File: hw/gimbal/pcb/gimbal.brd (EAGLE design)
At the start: 60 x 40 mm, 43 parts

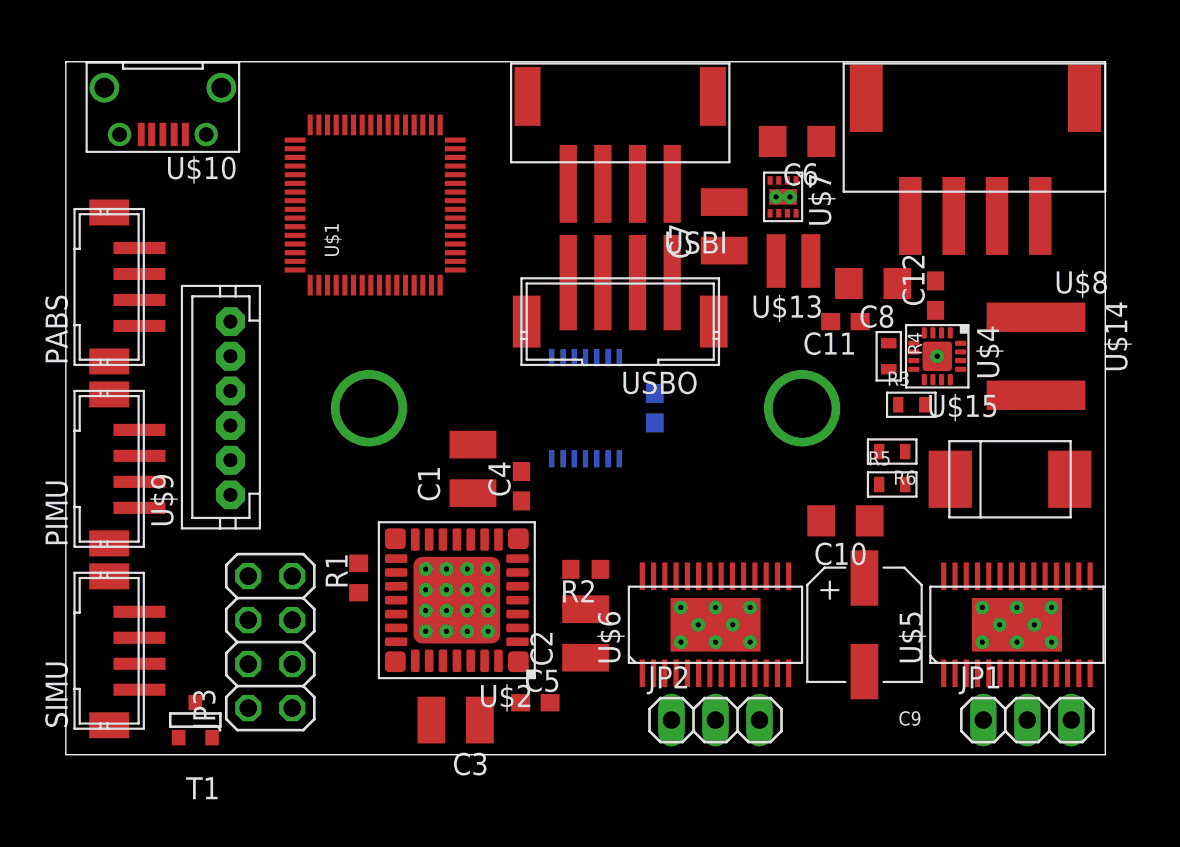
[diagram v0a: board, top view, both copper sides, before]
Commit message: Progress on gimbal board.
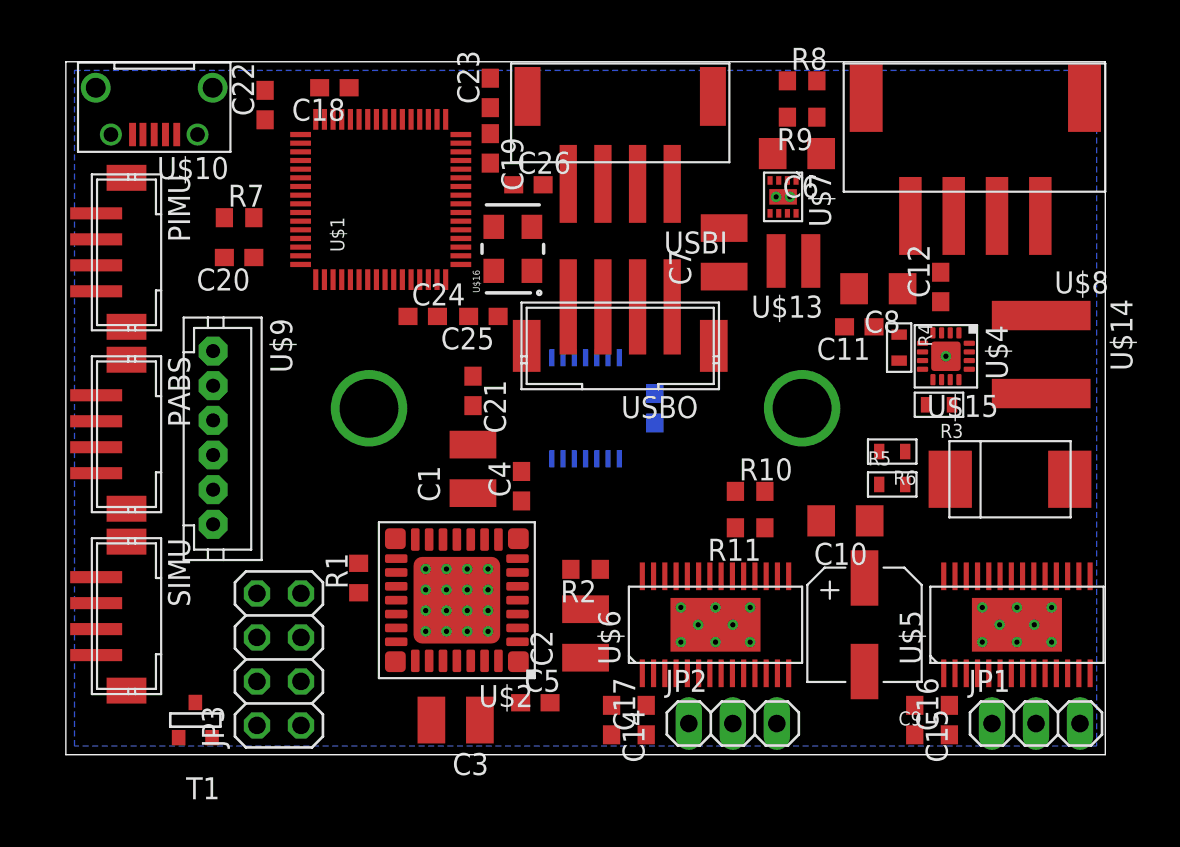
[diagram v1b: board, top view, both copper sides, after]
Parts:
- added C14, C15: 0.01uF, rcl:C0603
- added C16, C17, C20, C21, C22, C23, C24: 0.1uF, rcl:C0603
- added C18, C19: 4.7uF, rcl:C0603
- added C25, C26: 10pF, rcl:C0603
- added R10, R8: 100k, rcl:R0603
- added R11, R9: 10k, rcl:R0603
- added R7: 10, rcl:R0603
- added U$16: (no value), gimbal:CRYSTAL-OSC-SMD-5X3.2
- U$14: value (none) -> 2.2uH
- moved PIMU 12.5 mm to (2.50, 29.0), turned to 270 degrees
- moved PABS 8.56 mm to (2.50, 18.5), turned to 270 degrees
- moved SIMU 2.24 mm to (2.50, 8.00), turned to 270 degrees
- moved U$9 1.97 mm to (8.50, 18.3), turned to 270 degrees
- moved R3 1.60 mm to (50.4, 20.2), turned to 180 degrees
- moved C7 1.50 mm to (38.0, 29.0)
- moved USBO 1.40 mm to (32.0, 24.1)
- moved JP3 1.12 mm to (12.3, 5.50)
- moved JP2 1.02 mm to (38.5, 1.80)
- moved C11 0.85 mm to (45.8, 24.7)
- moved R4 0.78 mm to (48.1, 23.5)
- moved C6 0.70 mm to (42.2, 34.7)
- moved C12 0.58 mm to (50.5, 27.0)
- moved JP1 0.54 mm to (56.0, 1.80)
- moved U$10 0.50 mm to (5.10, 37.3)
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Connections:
- new net BLDC_FAULT1: U$1.51, U$5.18
- new net BLDC_FAULT2: U$1.40, U$6.18
- new net BLDC_RESET/: U$1.4, U$5.16, U$6.16
- new net BLDC_SLEEP/: U$1.3, U$5.17, U$6.17
- new net MOTOR1_EN: U$5.22, U$5.24, U$5.26
- new net MOTOR1_IN1: U$1.37, U$5.27
- new net MOTOR1_IN2: U$1.38, U$5.25
- new net MOTOR1_IN3: U$1.39, U$5.23
- new net MOTOR2_EN: U$6.22, U$6.24, U$6.26
- new net MOTOR2_IN1: U$1.14, U$6.27
- new net MOTOR2_IN2: U$1.15, U$6.25
- new net MOTOR2_IN3: U$1.16, U$6.23
- new net N$23: C18.1, U$1.30
- new net N$24: C24.1, U$1.7, U$9.5
- new net N$25: C14.1, U$6.1
- new net N$26: C14.2, U$6.2
- new net N$27: C15.2, U$5.2
- new net N$28: C15.1, U$5.1
- new net N$29: C16.2, U$5.3
- new net N$30: C17.2, U$6.3
- new net N$31: U$1.49, U$9.2
- new net N$32: U$1.46, U$9.4
- new net N$33: R7.2, U$1.60
- new net N$34: R8.1, R9.2, U$1.9
- new net N$35: C25.1, U$1.5, U$16.1
- new net N$36: C26.1, U$1.6, U$16.3
- new net N$38: R10.1, R11.2, U$1.10
- new net SLAVE_RX: U$1.55, U$8.3
- new net SLAVE_TX: U$1.50, U$8.2
- net +12V: now also C16.1, C17.1, R10.2, U$5.11, U$5.4, U$6.11, U$6.4
- net +3V3: now also C19.1, C20.1, C21.1, C22.1, C23.1, JP3.5, U$1.1, U$1.13, U$1.19, U$1.32, U$1.48, U$1.64, U$9.1
- net +8V: now also R8.2, U$8.4
- net AEG_PWM: now also U$1.26
- net AGITATOR_PWM: now also U$1.27
- net BOOST_EN: now also U$1.52
- net GND: now also C18.2, C19.2, C20.2, C21.2, C22.2, C23.2, C24.2, C25.2, C26.2, R11.1, R7.1, R9.1, U$1.31, U$1.47, U$16.2, U$16.4, U$5.10, U$5.14, U$5.20, U$5.28, U$5.6, U$5.7, U$5.G0, U$5.G1, U$5.G2, U$5.G3, U$5.G4, U$5.G5, U$5.G6, U$5.G7, U$5.G8, U$6.10, U$6.14, U$6.20, U$6.28, U$6.6, U$6.7, U$6.G0, U$6.G1, U$6.G2, U$6.G3, U$6.G4, U$6.G5, U$6.G6, U$6.G7, U$6.G8, U$8.1, U$9.3
- net LASER_EN: now also U$1.28
- net MOTOR_D1: now also U$1.53
- net MOTOR_FB: now also U$1.8
- net MOTOR_SF: now also U$1.2
- net PABS_SCL: now also U$1.41; no longer U$1.61
- net PABS_SDA: now also U$1.61; no longer U$1.62
- net PIMU_SCL: now also U$1.58; no longer U$1.41
- net PIMU_SDA: now also U$1.59; no longer U$1.40
- net SIMU_SDA: now also U$1.62; no longer U$1.55
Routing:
- added copper zone on layer 16, net GND
